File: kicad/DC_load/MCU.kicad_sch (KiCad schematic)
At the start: 118 parts, among them J1 BNC, J10 DC fan connector, J6 USB_B, J8 FT232 programming port, J9 Conn_01x04_Socket, Q1 MMBT5401, SW1 RotaryEncoder_Switch, SW2 RotaryEncoder_Switch, SW3 SW_Push, SW8 SW_Push, U1 FSA3157P6X, U10 FSA3157P6X, U11 FSA3157P6X, U12 FSA3157P6X, U14 AMS1117-3.3, U15 74HC14D653, U16 93LCxxB, U17 CH340C, U18 TL431DBZ, U2 Screen, U8 STM32F103C8Tx

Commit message: Schematic done.
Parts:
- removed C42, C43: 47p, Capacitor_SMD:C_0603_1608Metric_Pad1.08x0.95mm_HandSolder, symbol Device:C
- removed C44: 10n, Capacitor_SMD:C_0603_1608Metric_Pad1.08x0.95mm_HandSolder, symbol Device:C
- removed C48: 100n, Capacitor_SMD:C_0603_1608Metric_Pad1.08x0.95mm_HandSolder, symbol Device:C
- removed C57: 10u, Capacitor_SMD:C_0603_1608Metric_Pad1.08x0.95mm_HandSolder, symbol Device:C
- removed J6: USB_B, DC_load:62910416121, symbol Connector:USB_B
- removed R50: 100, Resistor_SMD:R_0603_1608Metric_Pad0.98x0.95mm_HandSolder, symbol Device:R
- removed TP1, TP5: TestPoint, TestPoint:TestPoint_Pad_D2.0mm, symbol Connector:TestPoint
- removed U17: CH340C, Package_SO:SOIC-16_3.9x9.9mm_P1.27mm, symbol DC_load:CH340C
- added J6: Iso board connector, Connector_PinSocket_2.54mm:PinSocket_1x07_P2.54mm_Vertical, symbol Connector:Conn_01x07_Pin
- added Q18: MMBT5401, Package_TO_SOT_SMD:SOT-23, symbol Transistor_BJT:MMBT3906
- added U4: LTV-817S, Package_DIP:SMDIP-4_W9.53mm, symbol Isolator:LTV-817S
- R48, R49: value 22 -> 1k; LCSC C23345 -> C22962
- R64: value 10k -> 1k; LCSC C25804 -> C22962
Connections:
- net 3V3: now also R49.1; no longer R64.1
- net FAN_PWM: no longer J10.4 (Pin_4)
- net GND: now also J6.4 (Pin_4), Q18.3 (C); no longer J10.1 (Pin_1)
- net FAN_PMW_5V: now reaches R48.2
- net FAN_PMW_5V: now also U4.4
- net at R49.2: now also U4.1
- net 5V_EXT: now reaches R48.1
- net 5V_EXT: now also J6.2 (Pin_2)
- net 12V renamed 12V_EXT
- net 12V_EXT: now also J6.3 (Pin_3); no longer TP6.1
- net 5V renamed VCC
- net VCC: now also TP6.1, J6.7 (Pin_7)
- net TACH: no longer names the net of R64.2
- net TACH: now also Q18.1 (B); no longer J10.3 (Pin_3)
- new net: Q18.2 (E), U4.2
- new net Earth: J10.1 (Pin_1), J6.1 (Pin_1), U4.3
- new net FAN_PMW: R64.1
- new net FAN_PWM_5V: J10.4 (Pin_4)
- new net RX_3V3: J6.6 (Pin_6)
- new net TX_3V3: J6.5 (Pin_5)
- no-connect marks 16 -> 10
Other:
- moved on the sheet: C16, C17, C18, C19, C30, C31, C32, C33, C34, C35, C45, C47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

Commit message: Replaced switches with JLCPCB basic.
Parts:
- SW3, SW8: footprint Button_Switch_THT:SW_TH_Tactile_Omron_B3F-10xx -> DC_load:TS-1088-AR02016; LCSC (none) -> C720477
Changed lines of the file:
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@@
 			)
 		)
-		(property "Footprint" "Button_Switch_THT:SW_TH_Tactile_Omron_B3F-10xx"
+		(property "Footprint" "DC_load:TS-1088-AR02016"
 			(at 196.85 43.18 0)
 			(effects
@@
 			)
 		)
+		(property "LCSC" "C720477"
+			(at 201.93 43.18 90)
+			(effects
+				(font
+					(size 1.27 1.27)
+				)
+				(hide yes)
+			)
+		)
 		(pin "2"
 		)
@@
 			)
 		)
-		(property "Footprint" "Button_Switch_THT:SW_TH_Tactile_Omron_B3F-10xx"
+		(property "Footprint" "DC_load:TS-1088-AR02016"
 			(at 167.64 60.96 0)
 			(effects
@@
 			(effects
 				(font
+					(size 1.27 1.27)
+				)
+				(hide yes)
+			)
+		)
+		(property "LCSC" "C720477"
+			(at 172.72 60.96 90)
+			(effects
+				(font

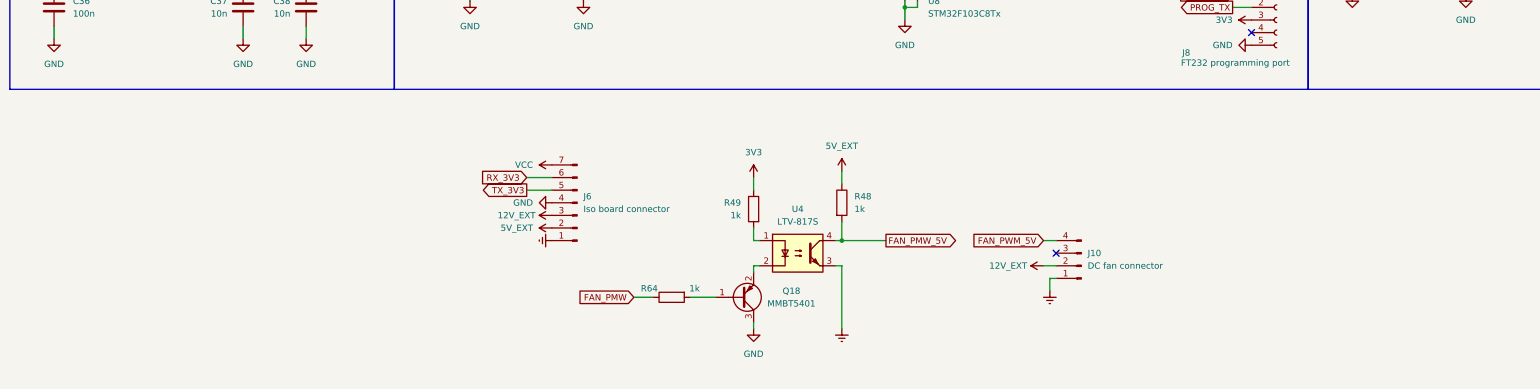
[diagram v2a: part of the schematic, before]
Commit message: Schem Schem.
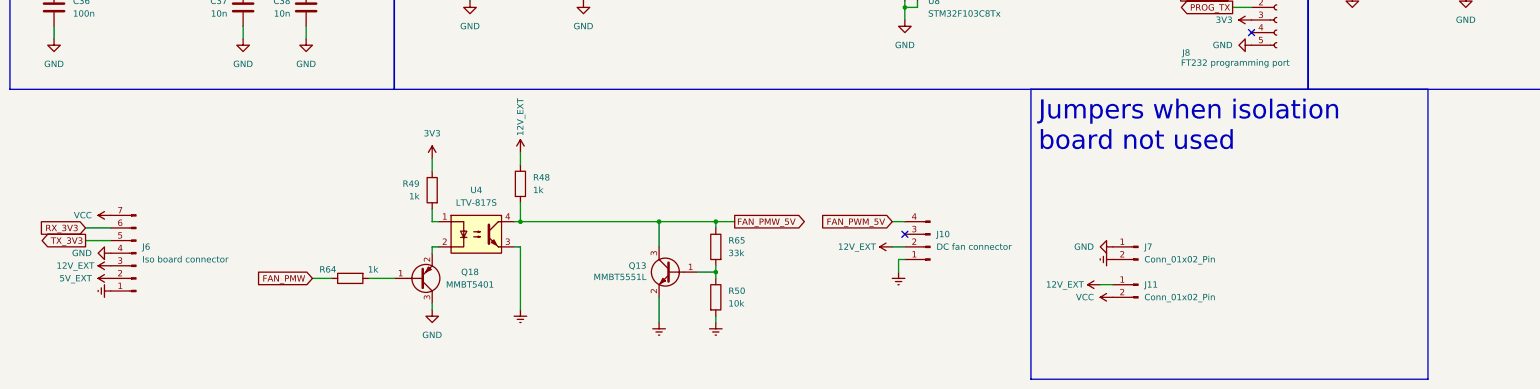
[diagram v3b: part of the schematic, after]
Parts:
- added J11, J7: Conn_01x02_Pin, Connector_PinHeader_2.54mm:PinHeader_1x02_P2.54mm_Vertical, symbol Connector:Conn_01x02_Pin
- added Q13: MMBT5551L, Package_TO_SOT_SMD:SOT-23, symbol Transistor_BJT:MMBT5551L
- added R50: 10k, Resistor_SMD:R_0603_1608Metric_Pad0.98x0.95mm_HandSolder, symbol Device:R
- added R65: 33k, Resistor_SMD:R_0603_1608Metric_Pad0.98x0.95mm_HandSolder, symbol Device:R
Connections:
- net 12V_EXT: now also R48.1, J11.1 (Pin_1)
- net 5V_EXT: no longer R48.1
- net Earth: now also J7.2 (Pin_2), Q13.2 (E), R50.2
- net FAN_PMW_5V: now also Q13.3 (C), R65.1
- net GND: now also J7.1 (Pin_1)
- net VCC: now also J11.2 (Pin_2)
- new net: Q13.1 (B), R50.1, R65.2
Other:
- note added: "Jumpers when isolation board not used"
- moved on the sheet: J10, J6, Q18, R48, R49, R64, U4
